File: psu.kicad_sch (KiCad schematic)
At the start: 8 parts, among them J2 USB_C_Receptacle_PowerOnly_6P, Q3 TIP125, Q4 TIP122

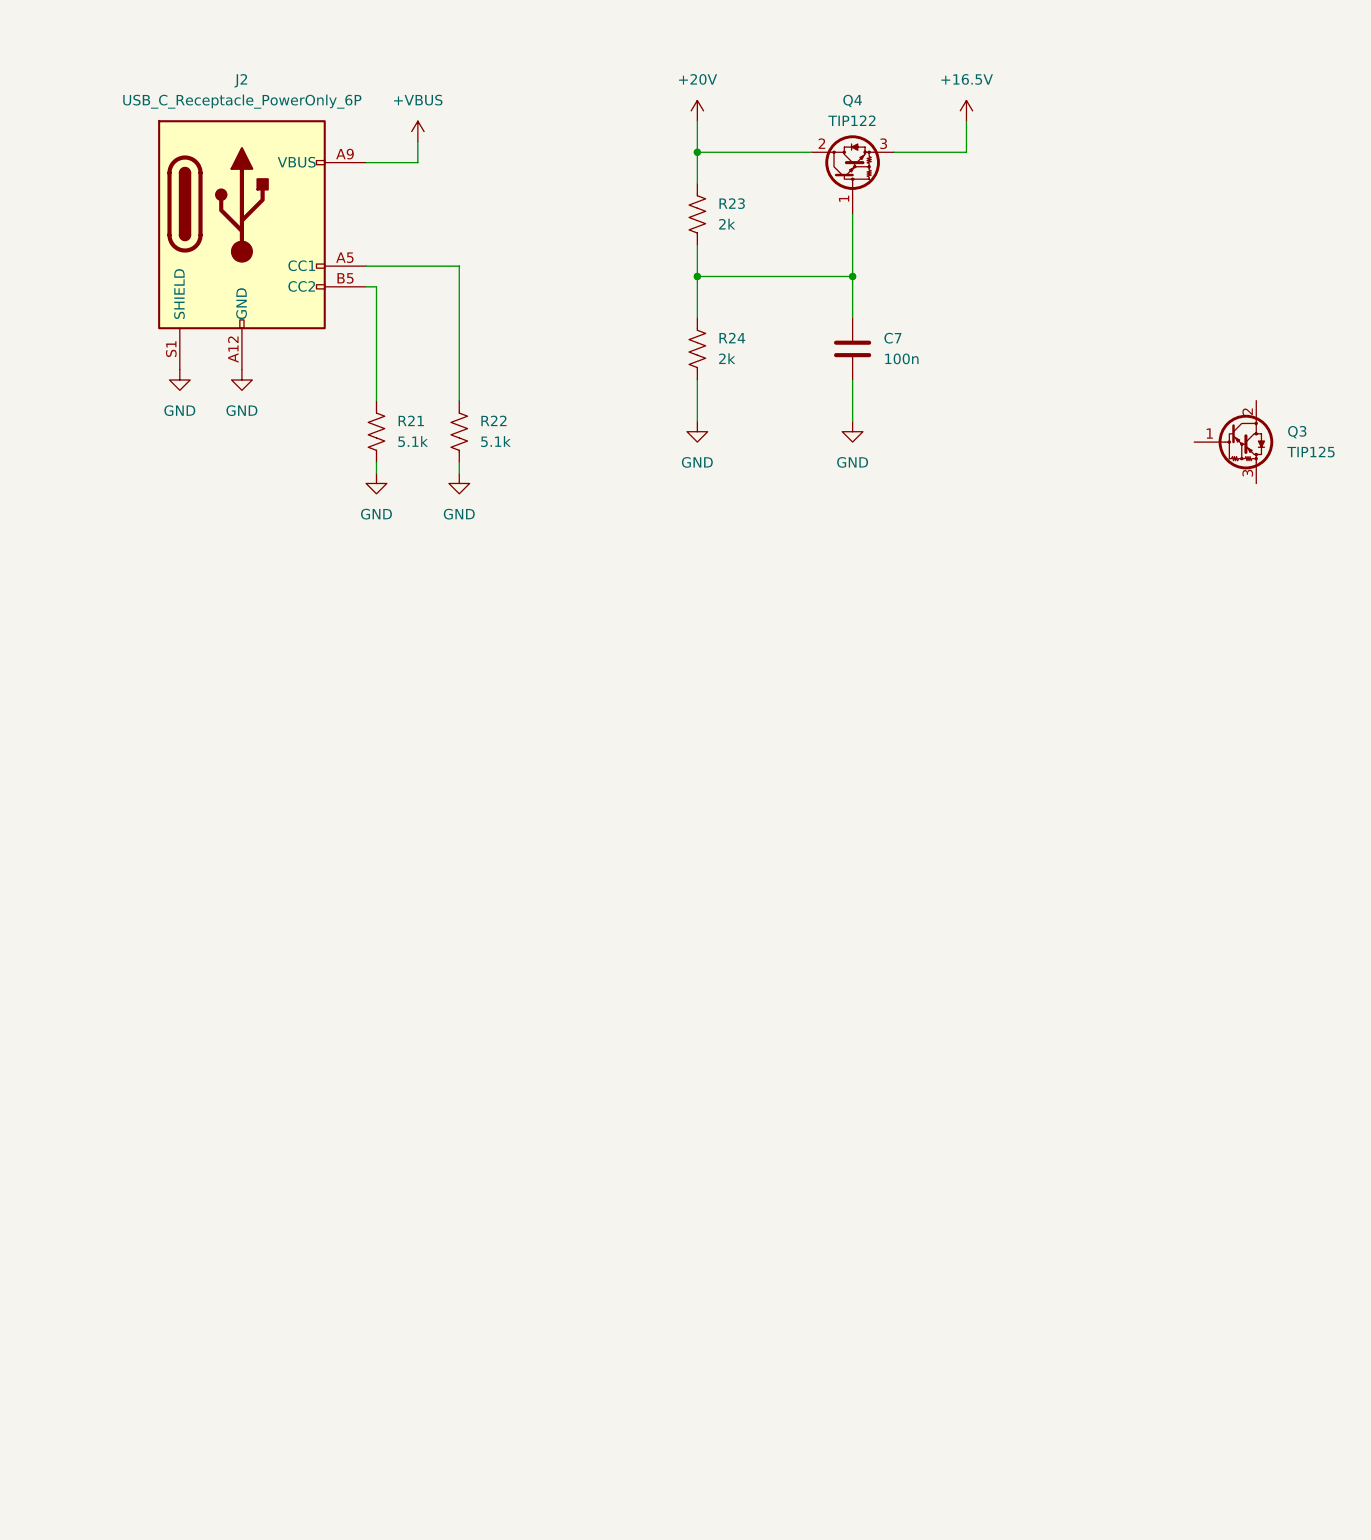
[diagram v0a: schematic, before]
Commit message: Progress.
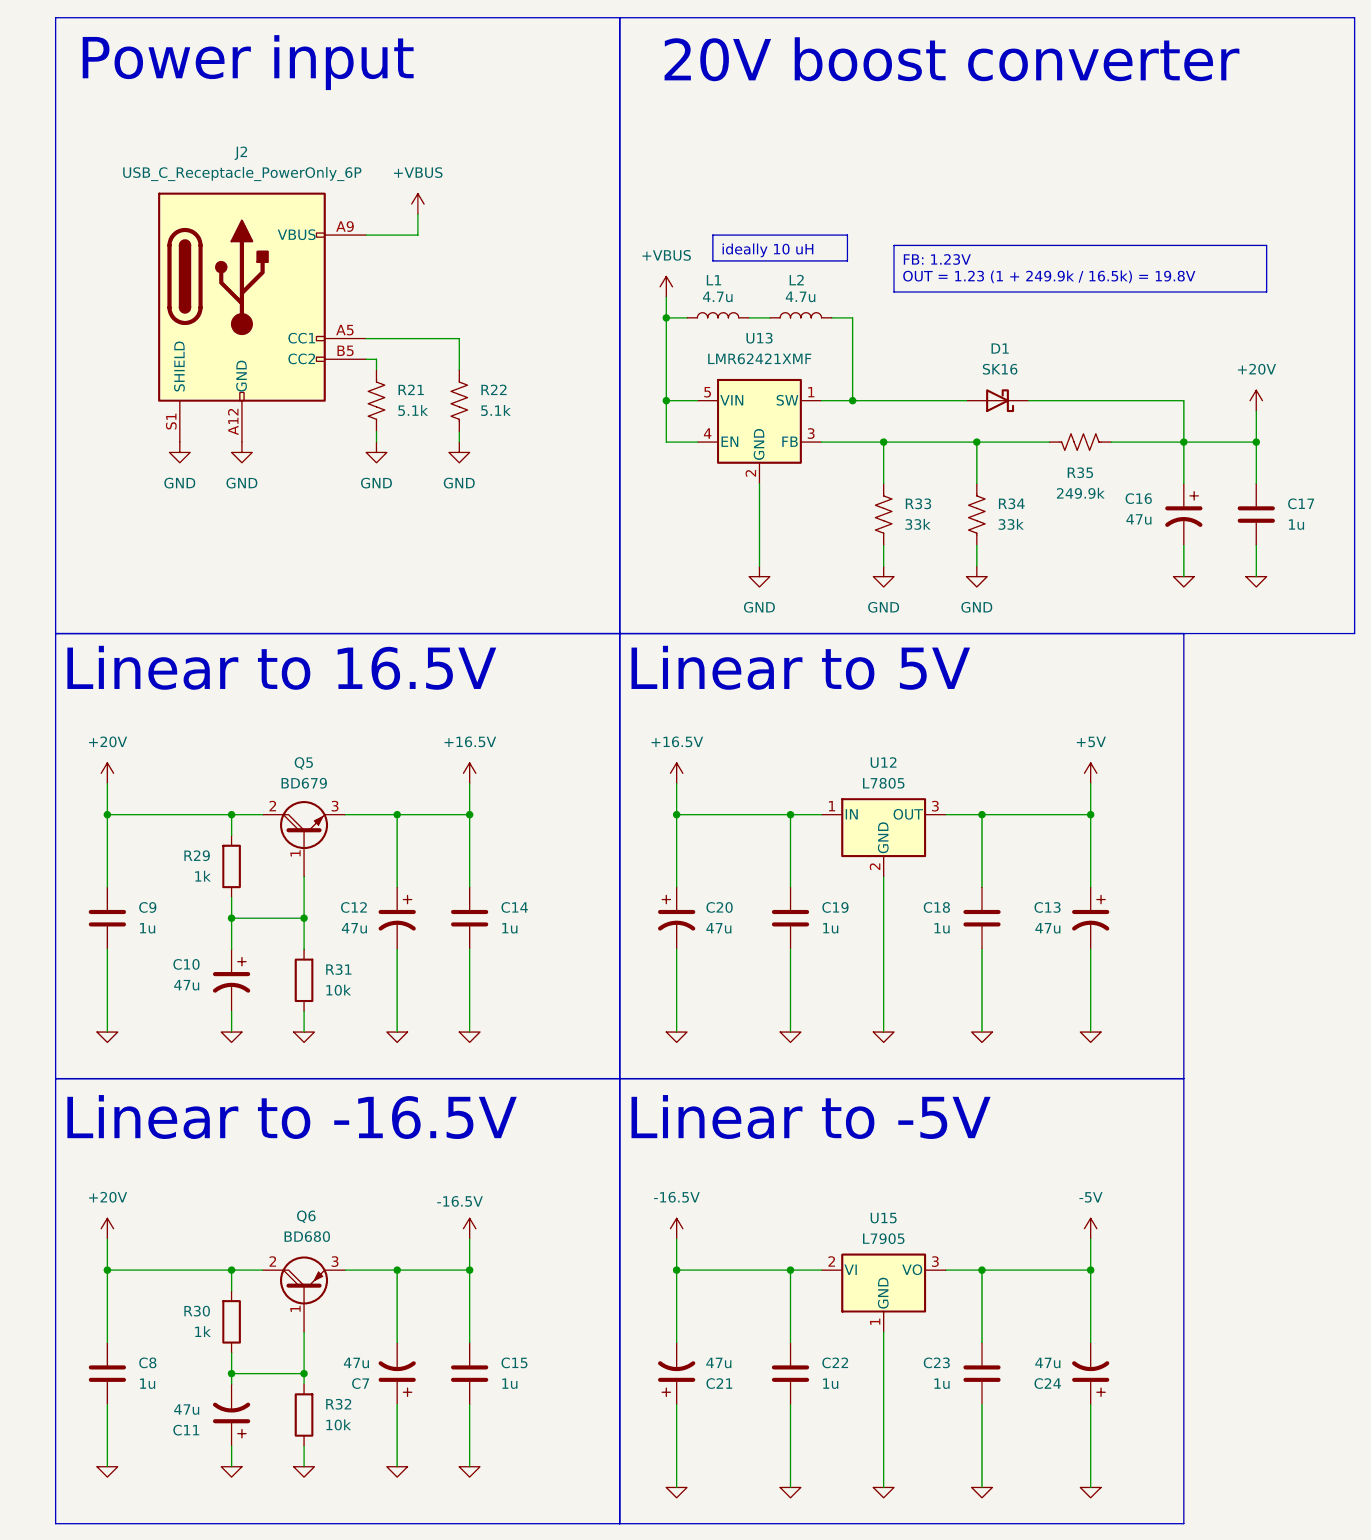
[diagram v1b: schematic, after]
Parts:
- removed C7: 100n, Capacitor_SMD:C_0603_1608Metric_Pad1.08x0.95mm_HandSolder, symbol Device:C
- removed Q3: TIP125, Package_TO_SOT_THT:TO-220-3_Vertical, symbol Transistor_BJT:TIP125
- removed Q4: TIP122, Package_TO_SOT_THT:TO-220-3_Vertical, symbol Transistor_BJT:TIP122
- removed R23, R24: 2k, Resistor_SMD:R_0603_1608Metric_Pad0.98x0.95mm_HandSolder, symbol Device:R_US
- added C10, C11, C12, C13, C16, C20, C21, C24, C7: 47u, Capacitor_THT:CP_Radial_D5.0mm_P2.00mm, symbol Device:C_Polarized_US
- added C14, C15, C17, C18, C19, C22, C23, C8, C9: 1u, Resistor_SMD:R_0603_1608Metric_Pad0.98x0.95mm_HandSolder, symbol Device:C
- added D1: SK16, Diode_SMD:D_SMA_Handsoldering, symbol solar_push_pull_sym_lib:SK16
- added L1, L2: 4.7u, Inductor_THT:L_Radial_D7.5mm_P3.50mm_Fastron_07P, symbol Device:L
- added Q5: BD679, Package_TO_SOT_THT:TO-126-3_Horizontal_TabUp, symbol DS100M06V_linear:BD679
- added Q6: BD680, Package_TO_SOT_THT:TO-126-3_Horizontal_TabUp, symbol DS100M06V_linear:BD680
- added R29, R30: 1k, Resistor_SMD:R_0603_1608Metric_Pad0.98x0.95mm_HandSolder, symbol Device:R
- added R31, R32: 10k, Resistor_SMD:R_0603_1608Metric_Pad0.98x0.95mm_HandSolder, symbol Device:R
- added R33, R34: 33k, Resistor_SMD:R_0603_1608Metric_Pad0.98x0.95mm_HandSolder, symbol Device:R_US
- added R35: 249.9k, Resistor_SMD:R_0603_1608Metric_Pad0.98x0.95mm_HandSolder, symbol Device:R_US
- added U12: L7805, symbol Regulator_Linear:L7805
- added U13: LMR62421XMF, Package_TO_SOT_SMD:SOT-23-5, symbol Regulator_Switching:LMR62421XMF
- added U15: L7905, symbol Regulator_Linear:L7905
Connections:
- net +16.5V: now also C12.1, C14.1, C19.1, C20.1, Q5.3 (E), U12.1 (IN)
- net +20V: now also C16.1, C17.1, C8.1, C9.1, D1.1 (K), Q5.2 (C), Q6.2 (C), R29.2, R30.2, R35.1
- net +VBUS: now also L1.1, U13.4 (EN), U13.5 (VIN)
- net GND: now also R33.1, R34.1, U13.2 (GND)
- new net: C10.1, Q5.1 (B), R29.1, R31.2
- new net: C11.2, Q6.1 (B), R30.1, R32.2
- new net: R33.2, R34.2, R35.2, U13.3 (FB)
- new net: D1.2 (A), L2.2, U13.1 (SW)
- new net: L1.2, L2.1
- new net +5V: C13.1, C18.1, U12.3 (OUT)
- new net -16.5V: C15.1, C21.2, C22.1, C7.2, Q6.3 (E), U15.2 (VI)
- new net -5V: C23.1, C24.2, U15.3 (VO)
- new net 0: C10.2, C11.1, C12.2, C13.2, C14.2, C15.2, C16.2, C17.2, C18.2, C19.2, C20.2, C21.1, C22.2, C23.2, C24.1, C7.1, C8.2, C9.2, R31.1, R32.1, U12.2 (GND), U15.1 (GND)
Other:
- note added: "20V boost converter"
- note added: "Linear to -16.5V"
- note added: "Linear to -5V"
- note added: "Linear to 16.5V"
- note added: "Linear to 5V"
- note added: "Power input"
- moved on the sheet: J2, R21, R22
